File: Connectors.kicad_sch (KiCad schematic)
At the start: 20 parts, among them J2 Conn_01x08_Male, J3 Conn_01x08_Male, J4 Conn_01x08_Male, J5 5V, J6 USB_C_Receptacle_USB2.0, U15 TPD4E02B04DQA

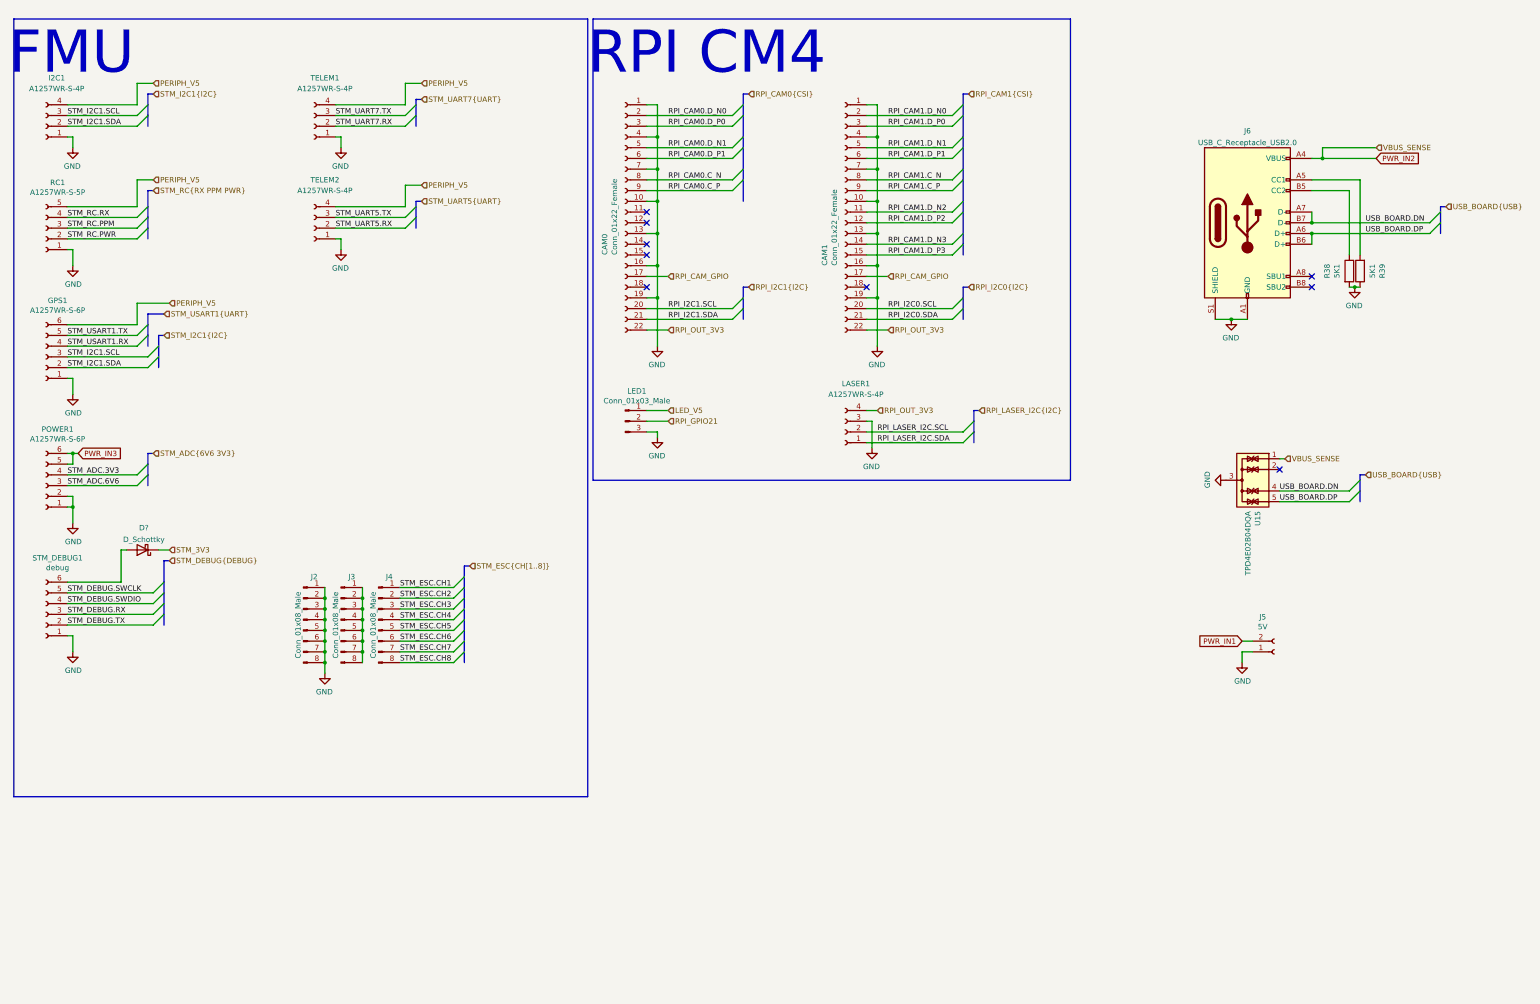
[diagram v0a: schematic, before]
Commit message: плата практически готова
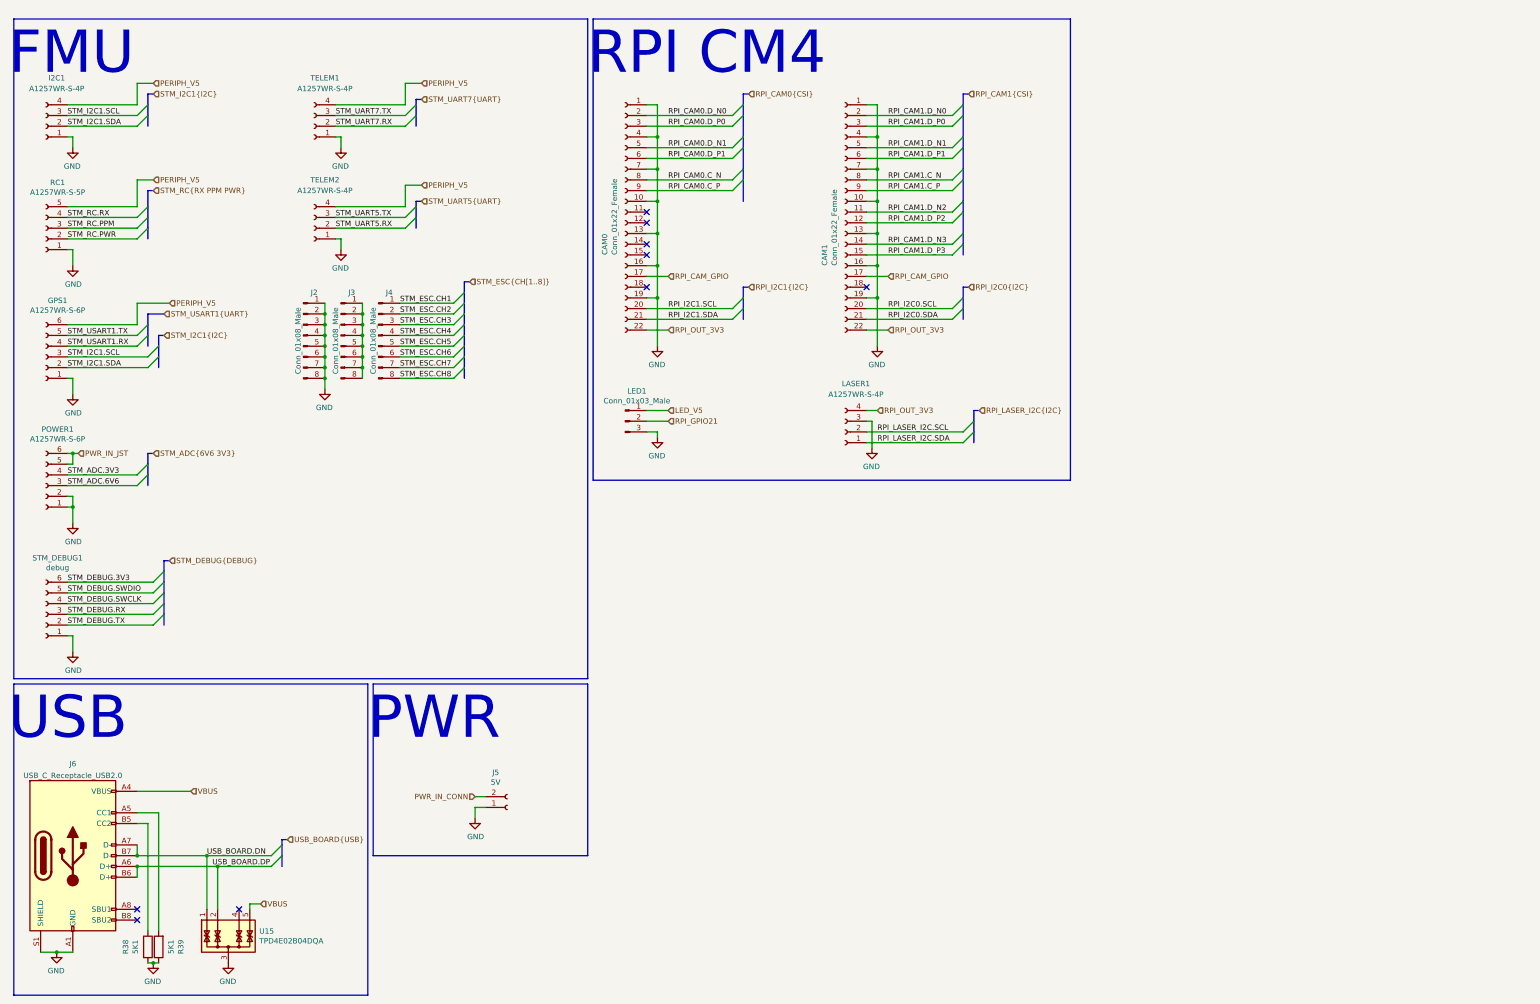
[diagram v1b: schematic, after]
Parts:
- removed D?: D_Schottky, Diode_SMD:D_0603_1608Metric, symbol Device:D_Schottky
- J6: footprint (none) -> Connector_USB:USB_C_Receptacle_HRO_TYPE-C-31-M-12; Manufacturer_Part_Number (none) -> 918-418K2023S40001
- STM_DEBUG1: footprint Connector:Tag-Connect_TC2030-IDC-NL_2x03_P1.27mm_Vertical -> Connector:debug_port
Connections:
- net STM_DEBUG.SWCLK: now also STM_DEBUG1.4 (Pin_4); no longer STM_DEBUG1.5 (Pin_5)
- net STM_DEBUG.SWDIO: now also STM_DEBUG1.5 (Pin_5); no longer STM_DEBUG1.4 (Pin_4)
- net USB_BOARD.DN: now also U15.1 (IO1); no longer U15.4 (IO3)
- net USB_BOARD.DP: now also U15.2 (IO2); no longer U15.5 (IO4)
- net STM_DEBUG.3V3: now reaches STM_DEBUG1.6 (Pin_6)
- net PWR_IN1 renamed PWR_IN_CONN
- net PWR_IN2 renamed VBUS
- net VBUS: now also U15.5 (IO4); no longer U15.1 (IO1)
- net PWR_IN3 renamed PWR_IN_JST
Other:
- note added: "PWR"
- note added: "USB"
- moved on the sheet: J2, J3, J4, J5, J6, R38, R39, U15
